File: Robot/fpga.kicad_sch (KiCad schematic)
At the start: 2 parts, among them U2 ICE40UP5K-SG48ITR, U3 74HCT245

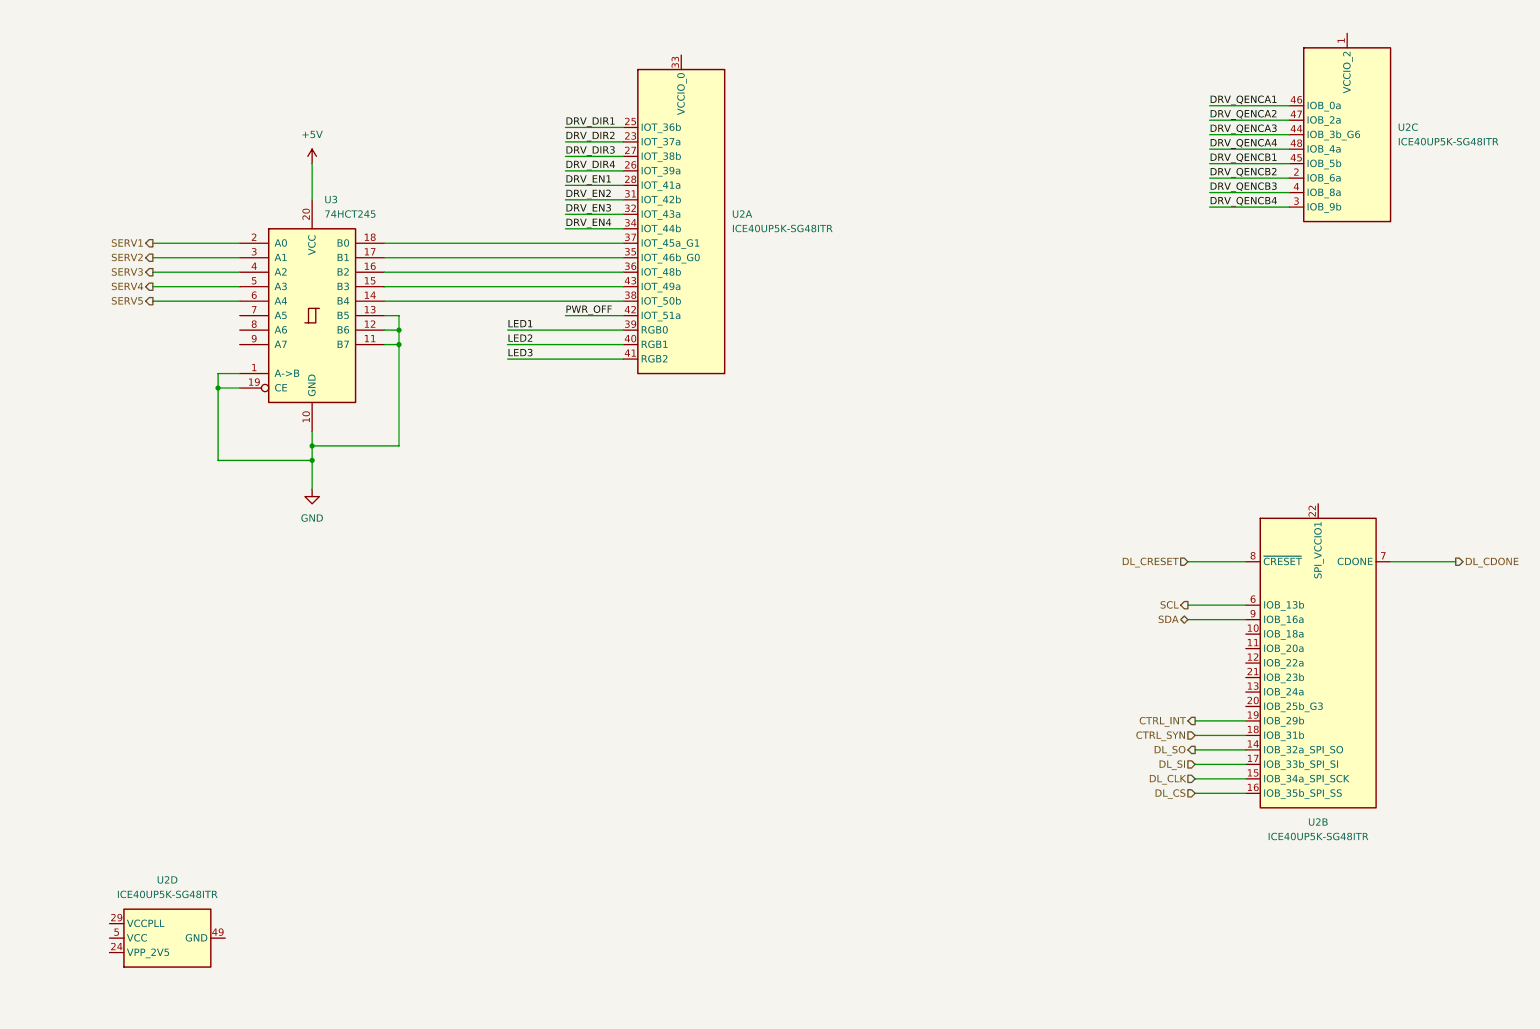
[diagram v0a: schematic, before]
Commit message: Update Robot SCH
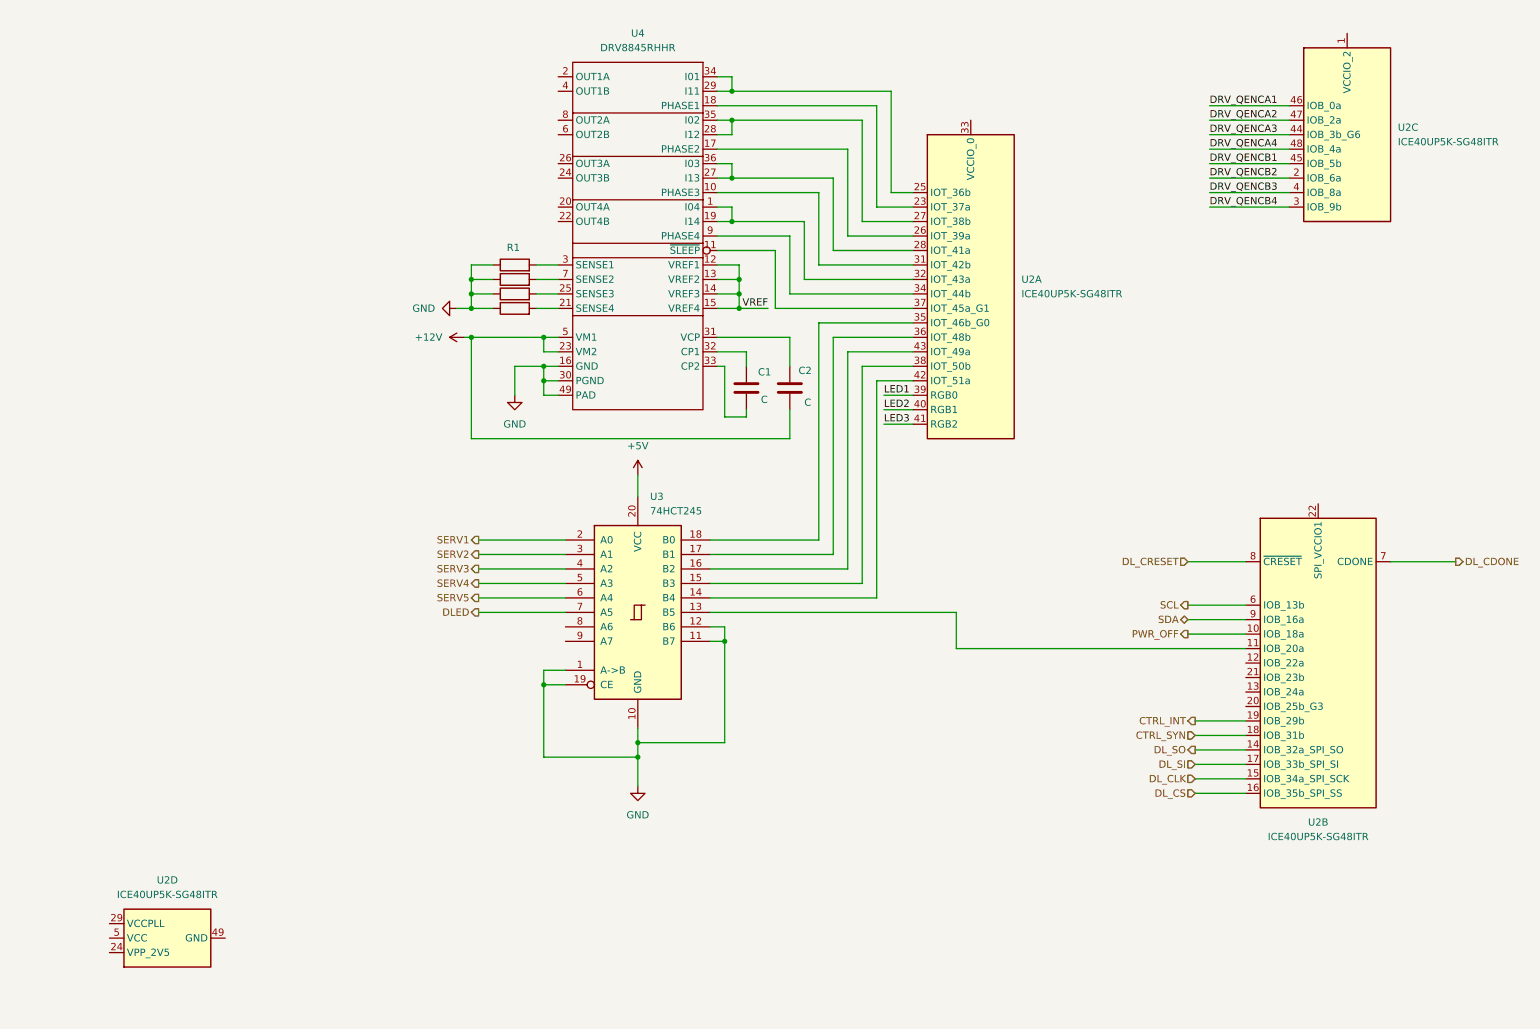
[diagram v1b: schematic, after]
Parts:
- added C1, C2: C, symbol Device:C
- added R1, R2, R3, R4: R, symbol Device:R
- added U4: DRV8845RHHR, symbol local:DRV8845
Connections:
- net GND: now also R1.1, R2.1, R3.1, R4.1, U4.16 (GND), U4.30 (PGND), U4.49 (PAD); no longer U3.13 (B5)
- net PWR_OFF: now also U2.10 (IOB_18a); no longer U2.42 (IOT_51a)
- net at U2.35 (IOT_46b_G0): now also U3.18 (B0); no longer U3.17 (B1)
- net at U2.36 (IOT_48b): now also U3.17 (B1); no longer U3.16 (B2)
- net at U2.37 (IOT_45a_G1): now also U4.11 (~{SLEEP}); no longer U3.18 (B0)
- net at U2.38 (IOT_50b): now also U3.15 (B3); no longer U3.14 (B4)
- net at U2.43 (IOT_49a): now also U3.16 (B2); no longer U3.15 (B3)
- net at U2.11 (IOB_20a): now also U3.13 (B5)
- net DLED: now reaches U3.7 (A5)
- net DRV_DIR1: no longer names the net of U2.25 (IOT_36b)
- net DRV_DIR1: now also U4.29 (I11), U4.34 (I01)
- net DRV_DIR2: no longer names the net of U2.23 (IOT_37a)
- net DRV_DIR2: now also U4.18 (PHASE1)
- net DRV_DIR3: no longer names the net of U2.27 (IOT_38b)
- net DRV_DIR3: now also U4.28 (I12), U4.35 (I02)
- net DRV_DIR4: no longer names the net of U2.26 (IOT_39a)
- net DRV_DIR4: now also U4.17 (PHASE2)
- net DRV_EN1: no longer names the net of U2.28 (IOT_41a)
- net DRV_EN1: now also U4.27 (I13), U4.36 (I03)
- net DRV_EN2: no longer names the net of U2.31 (IOT_42b)
- net DRV_EN2: now also U4.10 (PHASE3)
- net DRV_EN3: no longer names the net of U2.32 (IOT_43a)
- net DRV_EN3: now also U4.1 (I04), U4.19 (I14)
- net DRV_EN4: no longer names the net of U2.34 (IOT_44b)
- net DRV_EN4: now also U4.9 (PHASE4)
- new net: R2.2, U4.7 (SENSE2)
- new net: R1.2, U4.3 (SENSE1)
- new net: C2.1, U4.31 (VCP)
- new net: R4.2, U4.21 (SENSE4)
- new net: U2.42 (IOT_51a), U3.14 (B4)
- new net: R3.2, U4.25 (SENSE3)
- new net: C1.1, U4.32 (CP1)
- new net: C1.2, U4.33 (CP2)
- new net +12V: C2.2, U4.23 (VM2), U4.5 (VM1)
- new net VREF: U4.12 (VREF1), U4.13 (VREF2), U4.14 (VREF3), U4.15 (VREF4)
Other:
- moved on the sheet: U2A, U3

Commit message: Updated Robot SCH
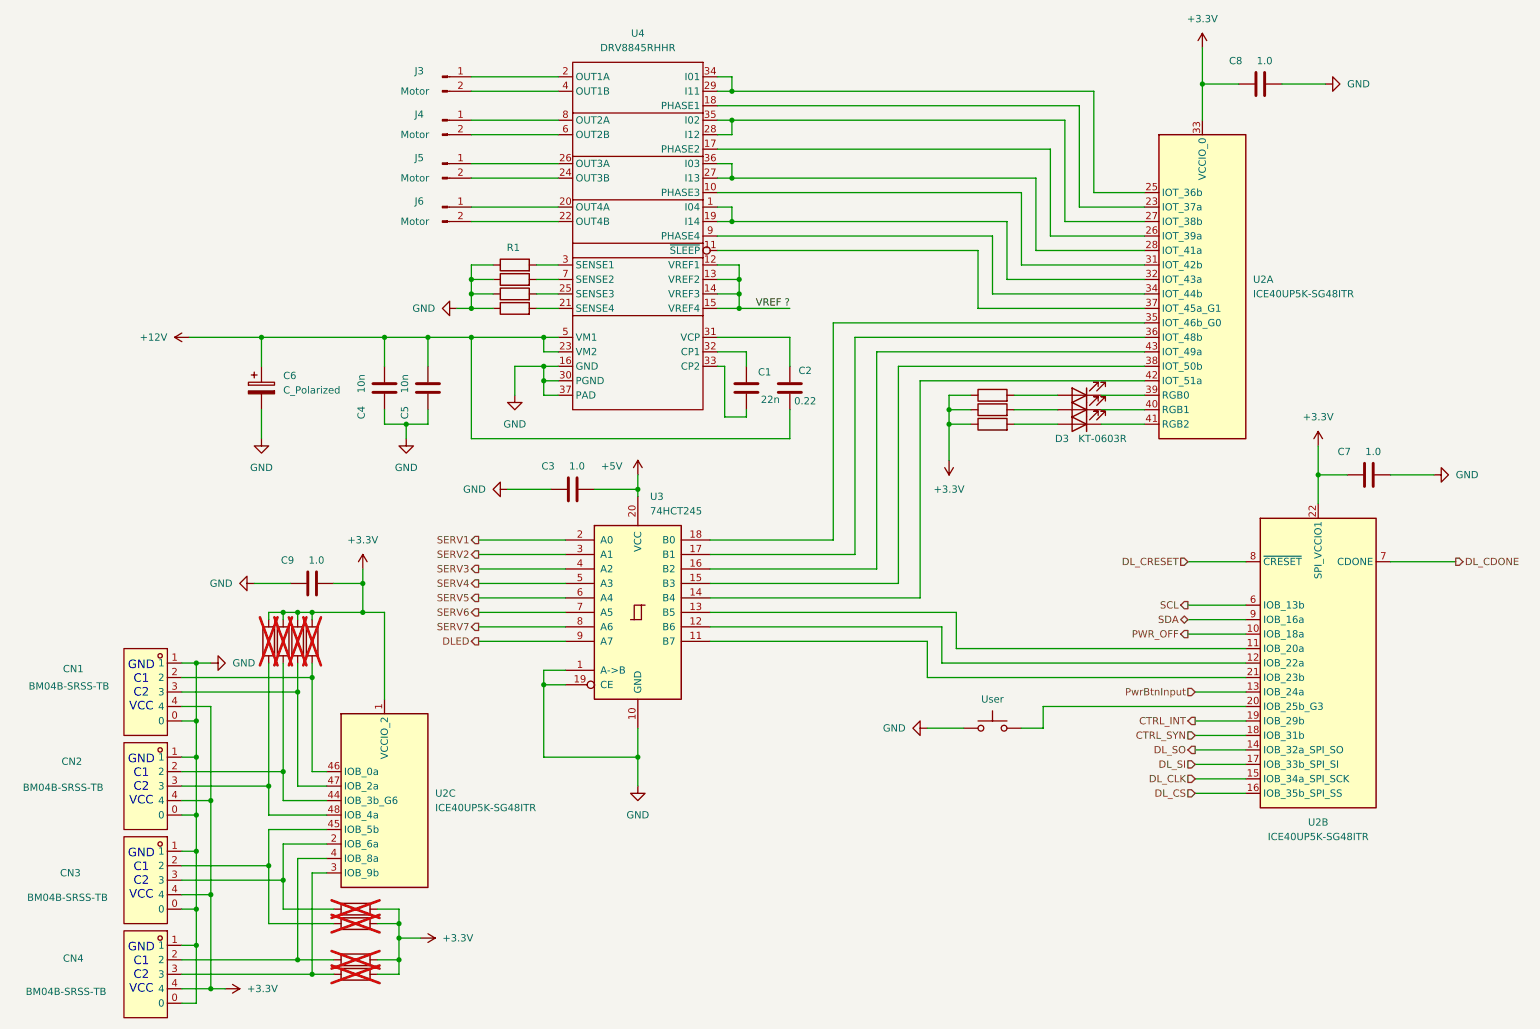
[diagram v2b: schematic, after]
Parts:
- removed unit 4 of U2
- added C3, C7, C8, C9: 1.0, symbol Device:C
- added C4, C5: 10n, symbol Device:C
- added C6: C_Polarized, symbol Device:C_Polarized
- added CN1, CN2, CN3, CN4: BM04B-SRSS-TB, easyeda2kicad:CONN-SMD_BM04B-SRSS-TB, symbol easyeda2kicad:BM04B-SRSS-TB
- added D1, D2, D3: KT-0603R, LED_SMD:LED_0603_1608Metric, symbol Device:LED
- added J3, J4, J5, J6: Motor, symbol Connector:Conn_01x02_Pin
- added R10, R11, R12, R13, R6, R7, R8, R9: NP, symbol Device:R
- added R14, R15, R16: R, symbol Device:R
- added SW2: User, symbol Switch:SW_Push
- C1: value C -> 22n
- C2: value C -> 0.22
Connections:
- net +12V: now also C4.2, C5.2, C6.1
- net +5V: now also C3.2
- net DLED: now also U3.9 (A7); no longer U3.7 (A5)
- net GND: now also U4.37 (PAD), C3.1, C4.1, C5.1, C6.2, C7.2, C8.2, C9.1, CN1.0, CN1.1, CN2.0, CN2.1, CN3.0, CN3.1, CN4.0, CN4.1, SW2.1; no longer U3.11 (B7), U3.12 (B6), U4.49 (PAD)
- net +3.3V: now reaches U2.33 (VCCIO_0)
- net +3.3V: now also U2.1 (VCCIO_2), U2.22 (SPI_VCCIO1), C7.1, C8.1, C9.2, CN1.4, CN2.4, CN3.4, CN4.4, R10.2, R11.2, R12.2, R13.2, R14.1, R15.1, R16.1, R6.2, R7.2, R8.2, R9.2
- net at U4.2 (OUT1A): now also J3.1 (Pin_1)
- net at U4.20 (OUT4A): now also J6.1 (Pin_1)
- net at U4.22 (OUT4B): now also J6.2 (Pin_2)
- net at U4.24 (OUT3B): now also J5.2 (Pin_2)
- net at U4.26 (OUT3A): now also J5.1 (Pin_1)
- net at U4.4 (OUT1B): now also J3.2 (Pin_2)
- net at U4.6 (OUT2B): now also J4.2 (Pin_2)
- net at U4.8 (OUT2A): now also J4.1 (Pin_1)
- net at U2.12 (IOB_22a): now also U3.12 (B6)
- net PwrBtnInput: now reaches U2.13 (IOB_24a)
- net at U2.20 (IOB_25b_G3): now also SW2.2
- net at U2.21 (IOB_23b): now also U3.11 (B7)
- net SERV7: now reaches U3.8 (A6)
- net DRV_QENCA1: no longer names the net of U2.46 (IOB_0a)
- net DRV_QENCA1: now also CN1.2, R11.1
- net DRV_QENCA2: no longer names the net of U2.47 (IOB_2a)
- net DRV_QENCA2: now also CN1.3, R10.1
- net DRV_QENCA3: no longer names the net of U2.44 (IOB_3b_G6)
- net DRV_QENCA3: now also CN2.2, R13.1
- net DRV_QENCA4: no longer names the net of U2.48 (IOB_4a)
- net DRV_QENCA4: now also CN2.3, R12.1
- net DRV_QENCB1: no longer names the net of U2.45 (IOB_5b)
- net DRV_QENCB1: now also CN3.2, R9.1
- net DRV_QENCB2: no longer names the net of U2.2 (IOB_6a)
- net DRV_QENCB2: now also CN3.3, R8.1
- net DRV_QENCB3: no longer names the net of U2.4 (IOB_8a)
- net DRV_QENCB3: now also CN4.2, R6.1
- net DRV_QENCB4: no longer names the net of U2.3 (IOB_9b)
- net DRV_QENCB4: now also CN4.3, R7.1
- net LED1: no longer names the net of U2.39 (RGB0)
- net LED1: now also D2.1 (K)
- net LED2: no longer names the net of U2.40 (RGB1)
- net LED2: now also D1.1 (K)
- net LED3: no longer names the net of U2.41 (RGB2)
- net LED3: now also D3.1 (K)
- net VREF renamed VREF ?
- new net: D2.2 (A), R14.2
- new net: D1.2 (A), R15.2
- new net: D3.2 (A), R16.2
- new net SERV6: U3.7 (A5)
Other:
- note added: "GND C1 C2 VCC"
- moved on the sheet: U2A, U2C
